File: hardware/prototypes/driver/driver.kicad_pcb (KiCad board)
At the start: 2 copper layers, 3 parts, among them Q1 AO3401A, U1 DRV8316CRRGFR, U2 PLMR36506RRPET

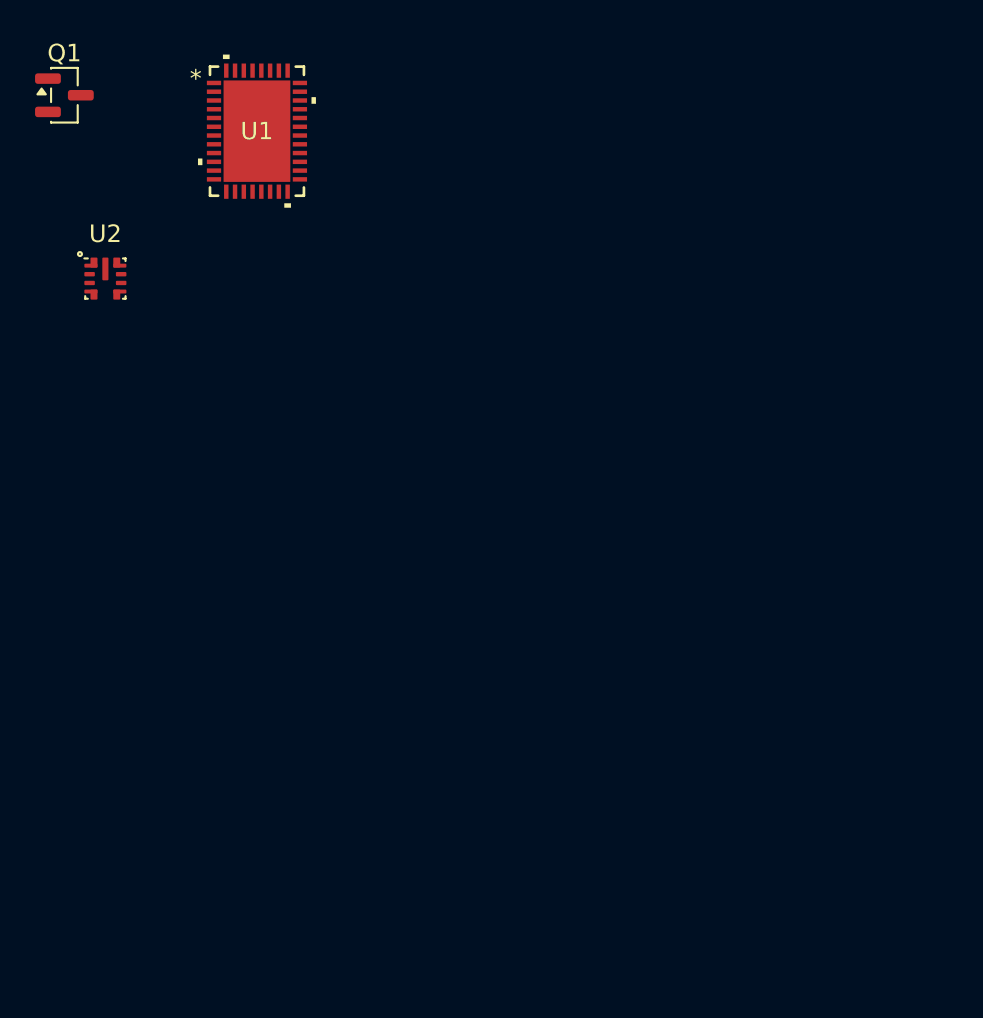
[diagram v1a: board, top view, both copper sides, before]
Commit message: fix: create fake prototype
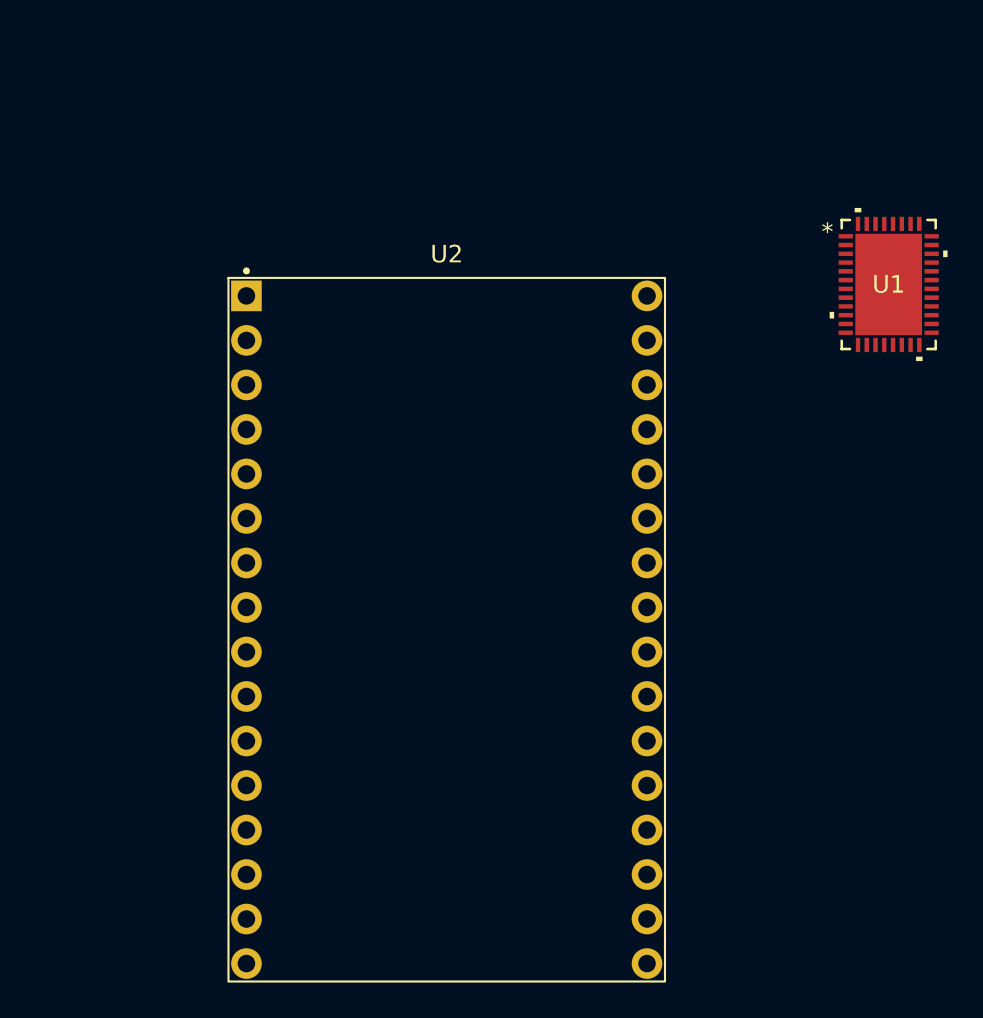
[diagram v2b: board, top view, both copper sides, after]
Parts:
- removed Q1: AO3401A, Package_TO_SOT_SMD:SOT-23
- U2: value PLMR36506RRPET -> ESP32-C6; footprint footprints:LMR36506 -> footprints:ESP32-C6-DevKitC-1_Socket
- moved U1 37.1 mm to (68.5, 36.2)
- moved U2 27.9 mm to (43.3, 56.0)
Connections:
- U1 pad 10: /VIN -> unconnected-(U1-VM-Pad10)
- U1 pad 11: /VIN -> unconnected-(U1-VM-Pad11)
- U1 pad 12: GND -> unconnected-(U1-PGND-Pad12)
- U1 pad 13: /OUTA -> unconnected-(U1-OUTA-Pad13)
- U1 pad 14: /OUTA -> unconnected-(U1-OUTA-Pad14)
- U1 pad 15: GND -> unconnected-(U1-PGND-Pad15)
- U1 pad 16: /OUTB -> unconnected-(U1-OUTB-Pad16)
- U1 pad 17: /OUTB -> unconnected-(U1-OUTB-Pad17)
- U1 pad 18: GND -> unconnected-(U1-PGND-Pad18)
- U1 pad 19: /OUTC -> unconnected-(U1-OUTC-Pad19)
- U1 pad 2: GND -> unconnected-(U1-AGND-Pad2)
- U1 pad 20: /OUTC -> unconnected-(U1-OUTC-Pad20)
- U1 pad 21: /DRVOFF -> unconnected-(U1-DRVOFF-Pad21)
- U1 pad 22: /NFAULT -> unconnected-(U1-NFAULT-Pad22)
- U1 pad 23: +3.3V -> unconnected-(U1-NSLEEP-Pad23)
- U1 pad 25: Net-(U1-AVDD) -> unconnected-(U1-AVDD-Pad25)
- U1 pad 26: GND -> unconnected-(U1-AGND-Pad26)
- U1 pad 27: /INHA -> unconnected-(U1-INHA-Pad27)
- U1 pad 28: /INLA -> unconnected-(U1-INLA-Pad28)
- U1 pad 29: /INHB -> unconnected-(U1-INHB-Pad29)
- U1 pad 3: /V_BUCK_OUT -> unconnected-(U1-FB_BK-Pad3)
- U1 pad 30: /INLB -> unconnected-(U1-INLB-Pad30)
- U1 pad 31: /INHC -> unconnected-(U1-INHC-Pad31)
- U1 pad 32: /INLC -> unconnected-(U1-INLC-Pad32)
- U1 pad 33: /SDO -> unconnected-(U1-SDO-Pad33)
- U1 pad 34: /SDI -> unconnected-(U1-SDI-Pad34)
- U1 pad 35: /CLK -> unconnected-(U1-SCLK-Pad35)
- U1 pad 36: /CS -> unconnected-(U1-NSCS-Pad36)
- U1 pad 37: Net-(U1-VREF/ILIM) -> unconnected-(U1-VREF/ILIM-Pad37)
- U1 pad 38: Net-(U1-SOC) -> unconnected-(U1-SOC-Pad38)
- U1 pad 39: Net-(U1-SOB) -> unconnected-(U1-SOB-Pad39)
- U1 pad 4: GND -> unconnected-(U1-GND_BK-Pad4)
- U1 pad 40: Net-(U1-SOA) -> unconnected-(U1-SOA-Pad40)
- U1 pad 41: GND -> unconnected-(U1-EPAD-Pad41)
- U1 pad 5: Net-(U1-SW_BK) -> unconnected-(U1-SW_BK-Pad5)
- U1 pad 6: Net-(U1-CPL) -> unconnected-(U1-CPL-Pad6)
- U1 pad 7: Net-(U1-CPH) -> unconnected-(U1-CPH-Pad7)
- U1 pad 8: Net-(U1-CP) -> unconnected-(U1-CP-Pad8)
- U1 pad 9: /VIN -> unconnected-(U1-VM-Pad9)
- U2 pad 1: Net-(U2-RT) -> unconnected-(U2-3V3-Pad1)
- U2 pad 3: /VIN -> unconnected-(U2-GPIO4/MTMS-Pad3)
- U2 pad 4: /VIN -> unconnected-(U2-GPIO5/MTDI-Pad4)
- U2 pad 5: Net-(U2-SW) -> unconnected-(U2-GPIO6-Pad5)
- U2 pad 6: Net-(U2-BOOT) -> unconnected-(U2-GPIO7-Pad6)
- U2 pad 7: Net-(U2-RT) -> unconnected-(U2-GPIO0-Pad7)
- U2 pad 8: +3.3V -> unconnected-(U2-GPIO1-Pad8)
- U2 pad 9: GND -> unconnected-(U2-GPIO8/BOOT-Pad9)
